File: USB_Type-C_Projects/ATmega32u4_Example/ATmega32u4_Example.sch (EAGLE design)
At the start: 49 parts, among them J1 105450-0101, J2 282834-3, J3 282834-3, J4 MF-CON-2.54mm-01x11, J5 MF-CON-2.54mm-01x11, SW1 MF-SW-TACT-4.2MM, U1 IP4234CZ6,125, U2 ATMEGA32U4-AU, X1 ABM3B-16.000MHZ-D-1-X-T

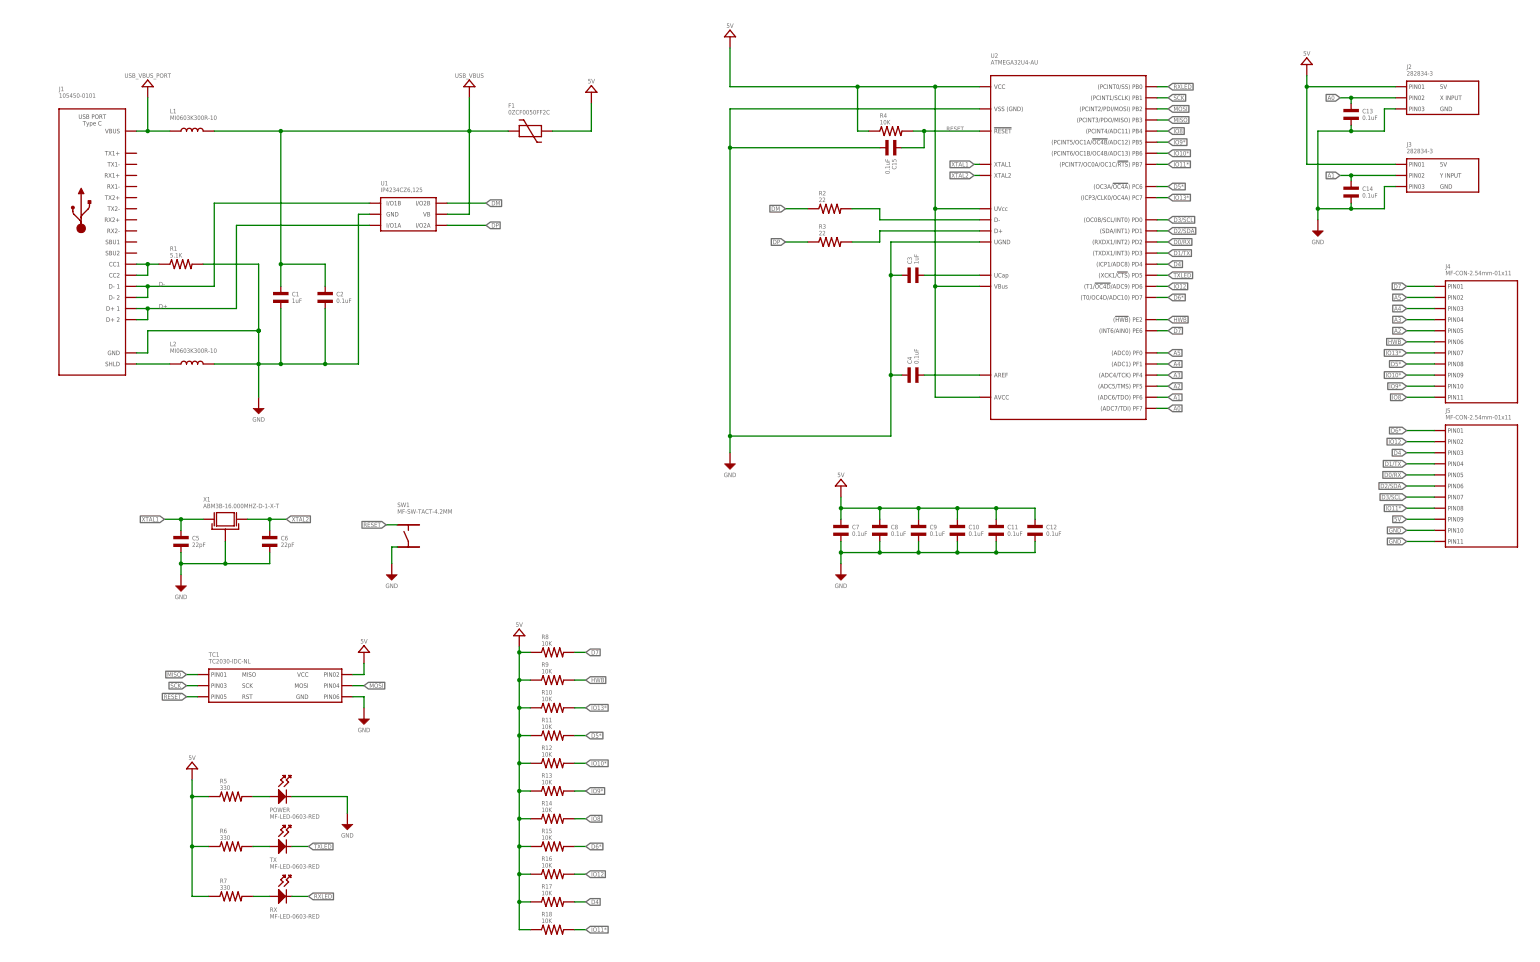
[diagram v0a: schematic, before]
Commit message: PCB complete. First rev ordered.
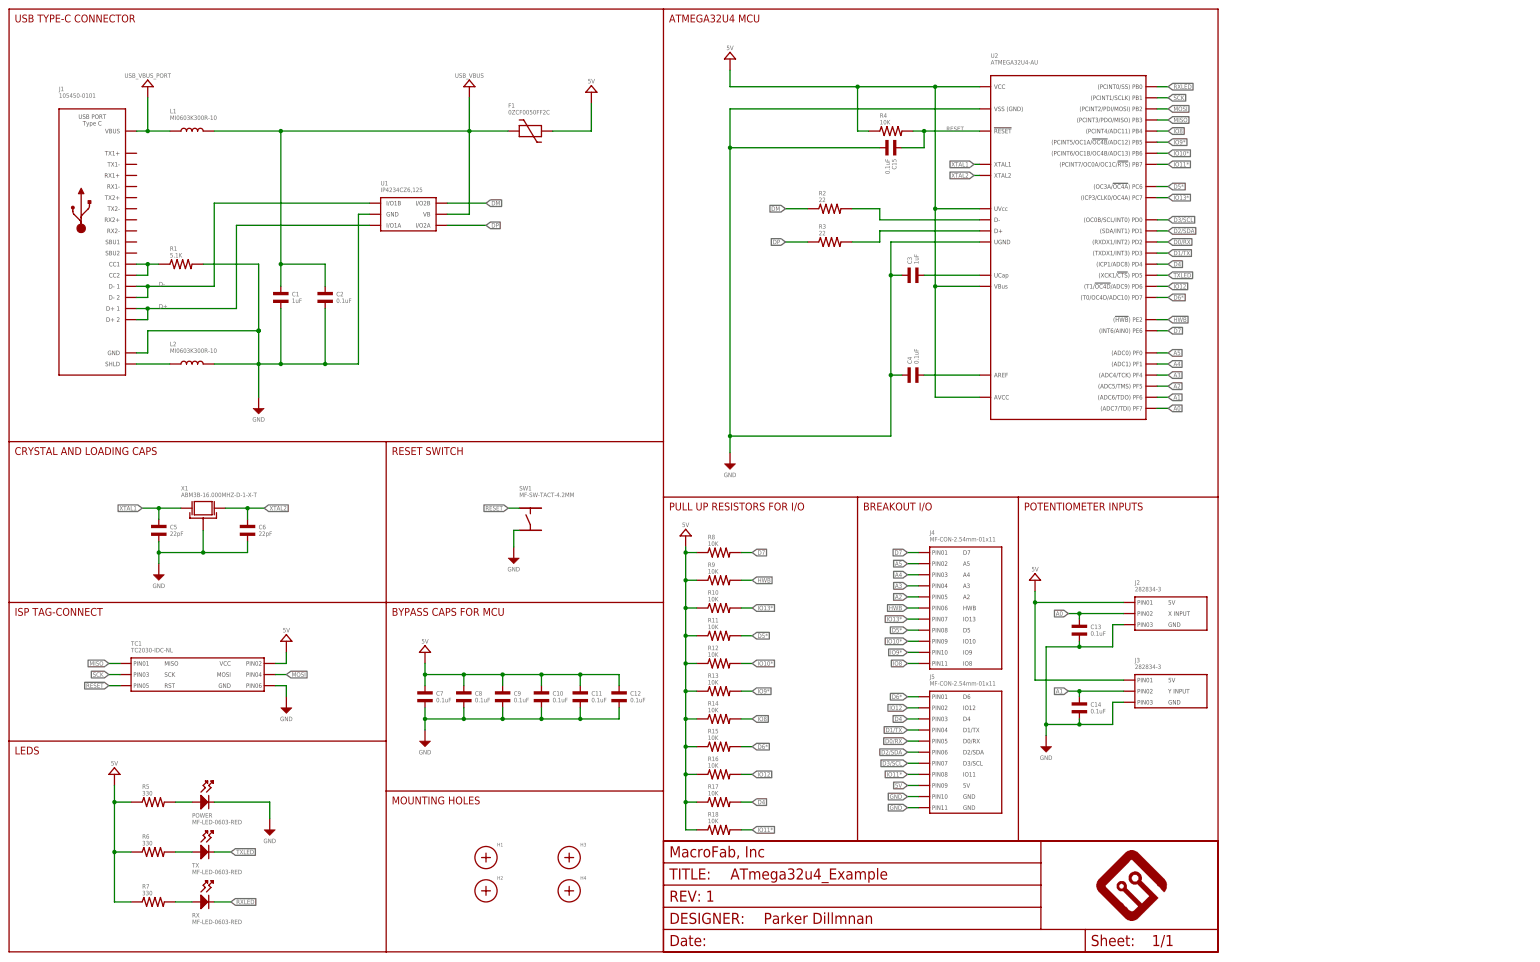
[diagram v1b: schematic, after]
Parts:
- added FRAME1: MF_FRAMEDEFAULT, MF_Aesthetics:MF_FRAMEDEFAULT
- added H1, H2, H3, H4: MOUNT_HOLE150MIL, PP_Connectors:MOUNT_HOLE150MIL
- J4: LABEL01 (none) -> D7; LABEL02 (none) -> A5; LABEL03 (none) -> A4; LABEL04 (none) -> A3; LABEL05 (none) -> A2; LABEL06 (none) -> HWB; LABEL07 (none) -> IO13; LABEL08 (none) -> D5; LABEL09 (none) -> IO10; LABEL10 (none) -> IO9; LABEL11 (none) -> IO8
- J5: LABEL01 (none) -> D6; LABEL02 (none) -> IO12; LABEL03 (none) -> D4; LABEL04 (none) -> D1/TX; LABEL05 (none) -> D0/RX; LABEL06 (none) -> D2/SDA; LABEL07 (none) -> D3/SCL; LABEL08 (none) -> IO11; LABEL09 (none) -> 5V; LABEL10 (none) -> GND; LABEL11 (none) -> GND
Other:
- note added: "ATMEGA32U4 MCU"
- note added: "BREAKOUT I/O"
- note added: "BYPASS CAPS FOR MCU"
- note added: "CRYSTAL AND LOADING CAPS"
- note added: "ISP TAG-CONNECT"
- note added: "LEDS"
- note added: "MOUNTING HOLES"
- note added: "POTENTIOMETER INPUTS"
- note added: "PULL UP RESISTORS FOR I/O"
- note added: "RESET SWITCH"
- note added: "USB TYPE-C CONNECTOR"
- moved on the sheet: C10, C11, C12, C13, C14, C5, C6, C7, C8, C9, J2, J3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
